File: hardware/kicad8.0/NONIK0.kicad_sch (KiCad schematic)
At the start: 26 parts, among them J1 AVR-UPDI-3, J2 Qwiic/Stemma QT, J3 Test Pads, J4 Test Pads, Q1 S8050, SW1 SW_SPST, SW2 SW_Push, SW3 SW_Push, U1 LED_HCMS-2915, U2 ATtiny1604-SS, U3 AP3602A

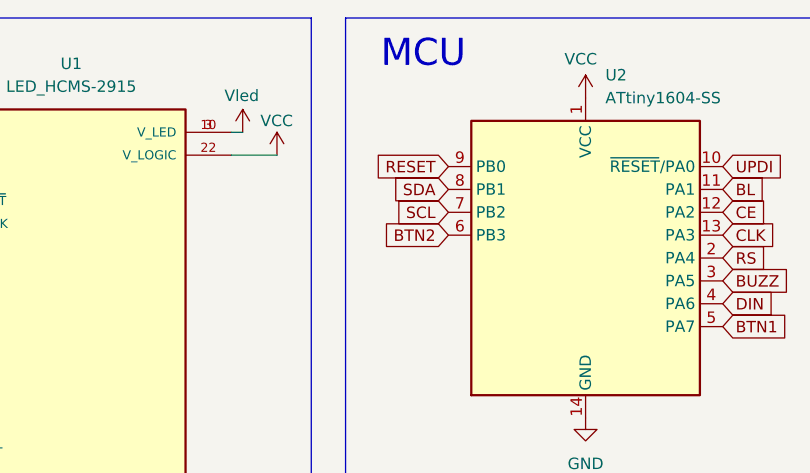
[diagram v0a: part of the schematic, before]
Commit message: pcb fixes, in progress
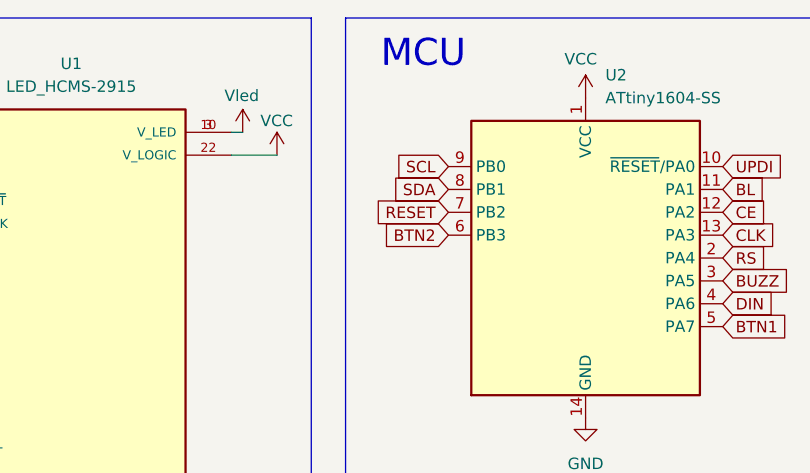
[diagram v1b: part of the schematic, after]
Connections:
- net RESET: now also U2.7 (PB2); no longer U2.9 (PB0)
- net SCL: now also U2.9 (PB0); no longer U2.7 (PB2)
